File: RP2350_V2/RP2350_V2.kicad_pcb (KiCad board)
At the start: 4 copper layers, 68.8 x 95.8 mm, 136 parts, among them IC1 DMP1045U-7, IC2 DMP1045U-7, IC3 DMP1045U-7, IC4 DMP1045U-7, J1 Conn_01x04_Pin, J2 901-143-6RFX, J3 USB_C_Receptacle_USB2.0_16P, J5 Conn_01x08_Socket, J6 Conn_01x02_Pin, J7 Conn_01x04_Pin, SW1 PTS 647 SN50 SMTR2 LFS, SW10 PTS 647 SN50 SMTR2 LFS, SW11 PTS 647 SN50 SMTR2 LFS, SW12 PTS 647 SN50 SMTR2 LFS, SW13 PTS 647 SN50 SMTR2 LFS, SW14 PTS 647 SN50 SMTR2 LFS, SW4 PTS 647 SN50 SMTR2 LFS, SW9 PTS 647 SN50 SMTR2 LFS, U1 RP2350_60QFN, U2 W25Q128JVS, U3 TPS62811QWRWYRQ1, U4 MCP73812T-420I-OT, U5 TLV3012AIDCKR, U6 74HC14, X1 ABM8-272-T3

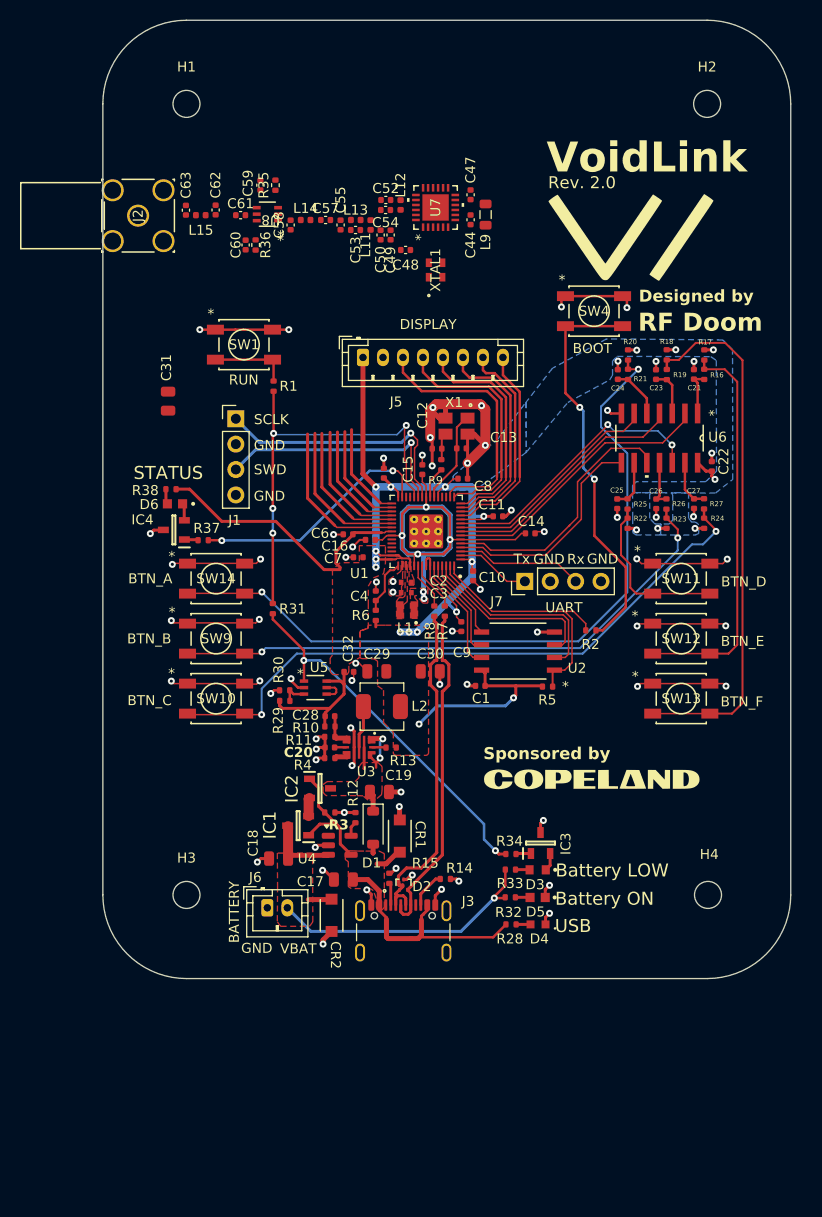
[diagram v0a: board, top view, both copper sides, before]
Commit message: progress :D
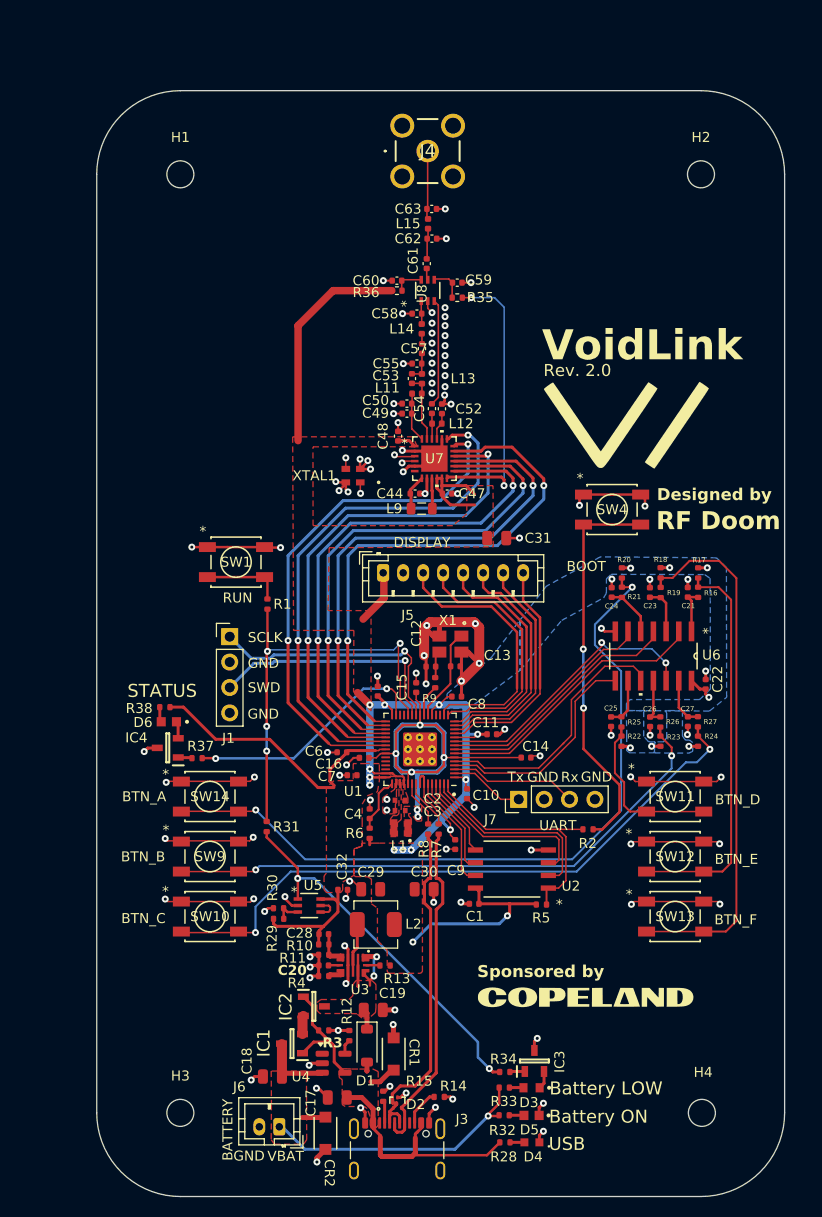
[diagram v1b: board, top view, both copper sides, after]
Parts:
- removed J2: 901-143-6RFX, My_Footprints:RF_ANT_OUTPUT_901-143-6RFX
- added J4: RF_CONNECTOR_5-1814832-2, My_Footprints:RF_CONNECTOR_518148322, F.Cu at (145.0, 44.5)
- moved C31 35.6 mm to (151.9, 83.2), turned to 0 degrees
- moved L9 30.1 mm to (144.4, 80.3), turned to 0 degrees
- moved C47 30.0 mm to (146.9, 78.8), turned to 180 degrees
- moved C44 27.9 mm to (143.7, 78.8), turned to 180 degrees
- moved U7 25.1 mm to (145.6, 75.3), turned to 0 degrees
- moved C63 24.6 mm to (145.4, 50.3), turned to 180 degrees
- moved L15 22.7 mm to (145.0, 51.8), turned to 90 degrees
- moved C14 22.4 mm to (154.8, 105.2)
- moved L12 22.2 mm to (145.9, 71.8), turned to 180 degrees
- moved XTAL1 22.2 mm to (137.5, 77.0), turned to 180 degrees
- moved C59 22.0 mm to (147.9, 57.7), turned to 0 degrees
- moved J6 21.9 mm to (130.1, 142.1), turned to 180 degrees
- moved C62 21.8 mm to (145.4, 53.3), turned to 180 degrees
- moved C11 21.8 mm to (151.4, 102.9)
- moved C19 21.8 mm to (139.5, 130.4)
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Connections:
- J6 pad 1: GND -> /VBAT
- J6 pad 2: /VBAT -> GND
- U1 pad 31: /SPI0_TX -> SPI0_TX
- U1 pad 32: /uC_RESET -> uC_RESET
- U1 pad 33: /uC_BUSY -> uC_BUSY
- U1 pad 34: /DIO1 -> DIO1
- U1 pad 35: /SPI0_RX -> SPIO_RX
- U1 pad 36: /CS/NSS -> CS/NSS
- U1 pad 37: /SPI0_CLK -> SPIO_CLK
- U7 pad 13: /SX1262/DIO1 -> DIO1
- U7 pad 14: /SX1262/BUSY -> uC_BUSY
- U7 pad 15: /SX1262/SX_NRESET -> uC_RESET
- U7 pad 16: /SX1262/MISO -> SPIO_RX
- U7 pad 17: /SX1262/MOSI -> SPI0_TX
- U7 pad 18: /SX1262/SCK -> SPIO_CLK
- U7 pad 19: /SX1262/NSS -> CS/NSS
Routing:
- net CS/NSS: track 0.00 -> 53.8 mm, vias 0 -> 2
- net SPI0_TX: track 0.00 -> 53.2 mm, vias 0 -> 2
- net uC_RESET: track 0.00 -> 52.4 mm, vias 0 -> 2
- net uC_BUSY: track 0.00 -> 52.1 mm, vias 0 -> 2
- net SPIO_CLK: track 0.00 -> 52.0 mm, vias 0 -> 2
- net DIO1: track 0.00 -> 52.0 mm, vias 0 -> 2
- net SPIO_RX: track 0.00 -> 51.6 mm, vias 0 -> 2
- net GND: track 161.5 -> 191.3 mm, vias 70 -> 110
- net +3V3: track 149.9 -> 179.2 mm
- net /SX1262/DIO2: track 0.00 -> 28.9 mm, vias 0 -> 2
- net /SPI0_CLK: track 16.1 -> 0.00 mm
- net /CS/NSS: track 15.2 -> 0.00 mm
- net /SPI0_RX: track 13.7 -> 0.00 mm
- net /DIO1: track 12.7 -> 0.00 mm
- net /uC_BUSY: track 11.6 -> 0.00 mm
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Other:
- board size 68.8 x 95.8 mm -> 68.8 x 110.6 mm
